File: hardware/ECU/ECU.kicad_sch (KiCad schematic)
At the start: 75 parts, among them IC1 IR4427SPBF, IC2 EL357NB_TA_-G, IC3 EL357NB_TA_-G, J1 USB_B_Micro, J2 TFP09-2-12B, J3 Connector, Q1 S8050, Q2 S8050, Q3 RJP63K2, Q4 RJP63K2, SW1 RESET, SW2 EN, U1 AMS1117-3.3, U2 AMS1117-3.3, U3 CP2102N-Axx-xQFN28, U4 ESP32-WROOM-32U

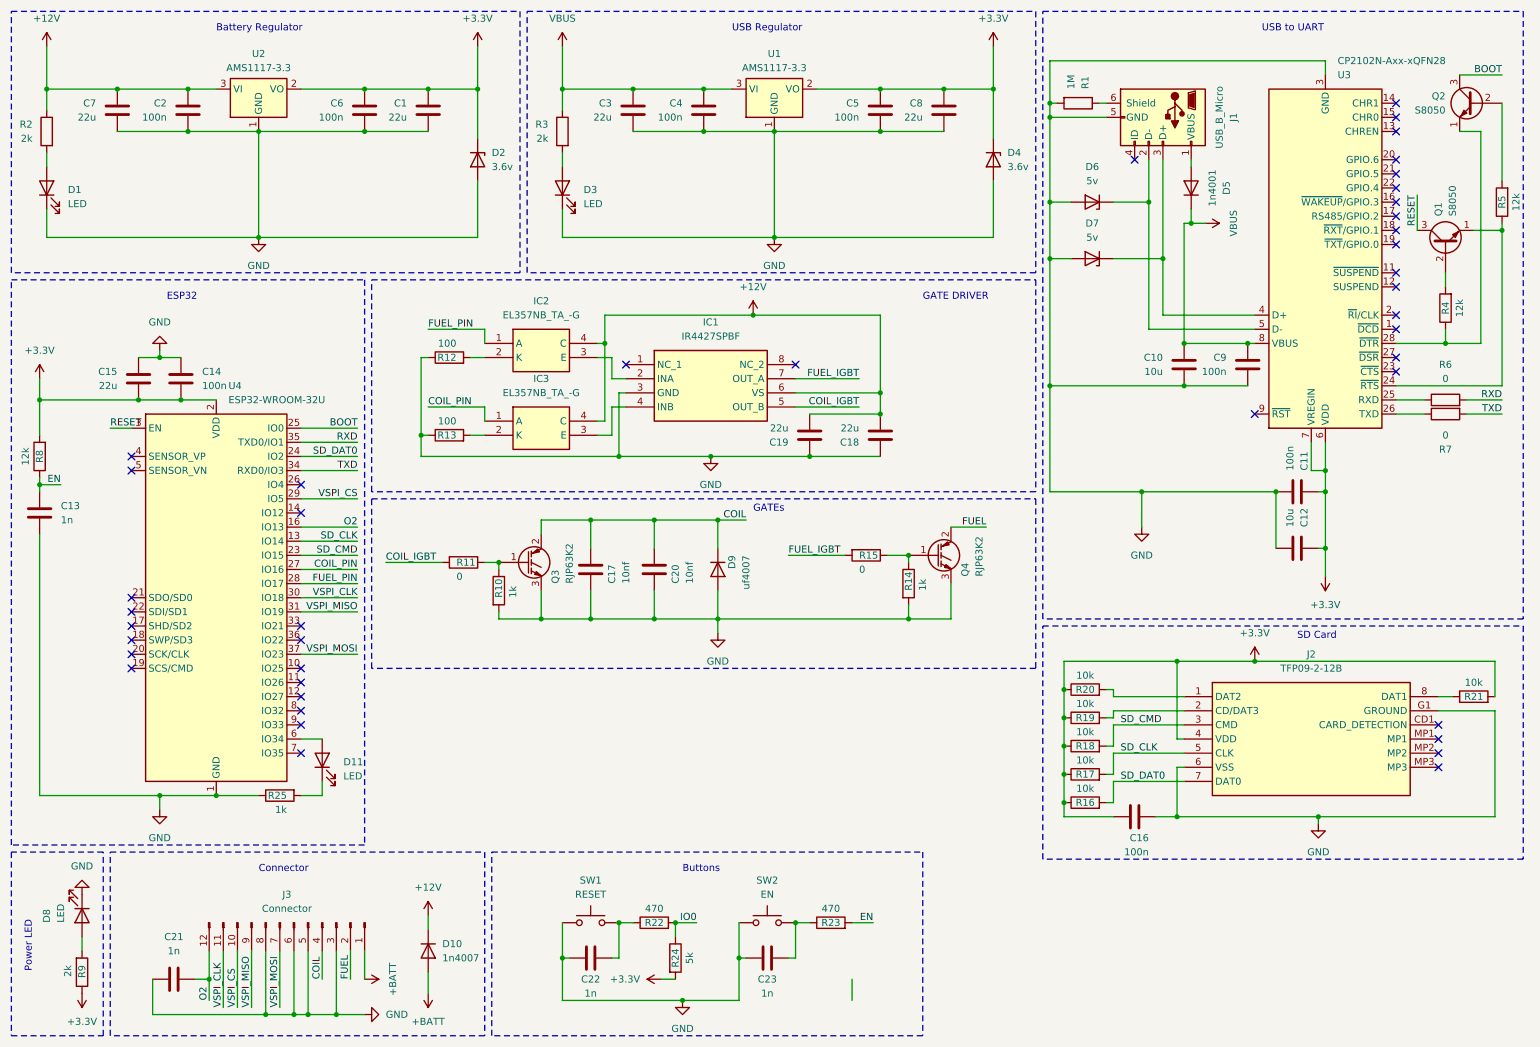
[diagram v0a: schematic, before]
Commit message: backup
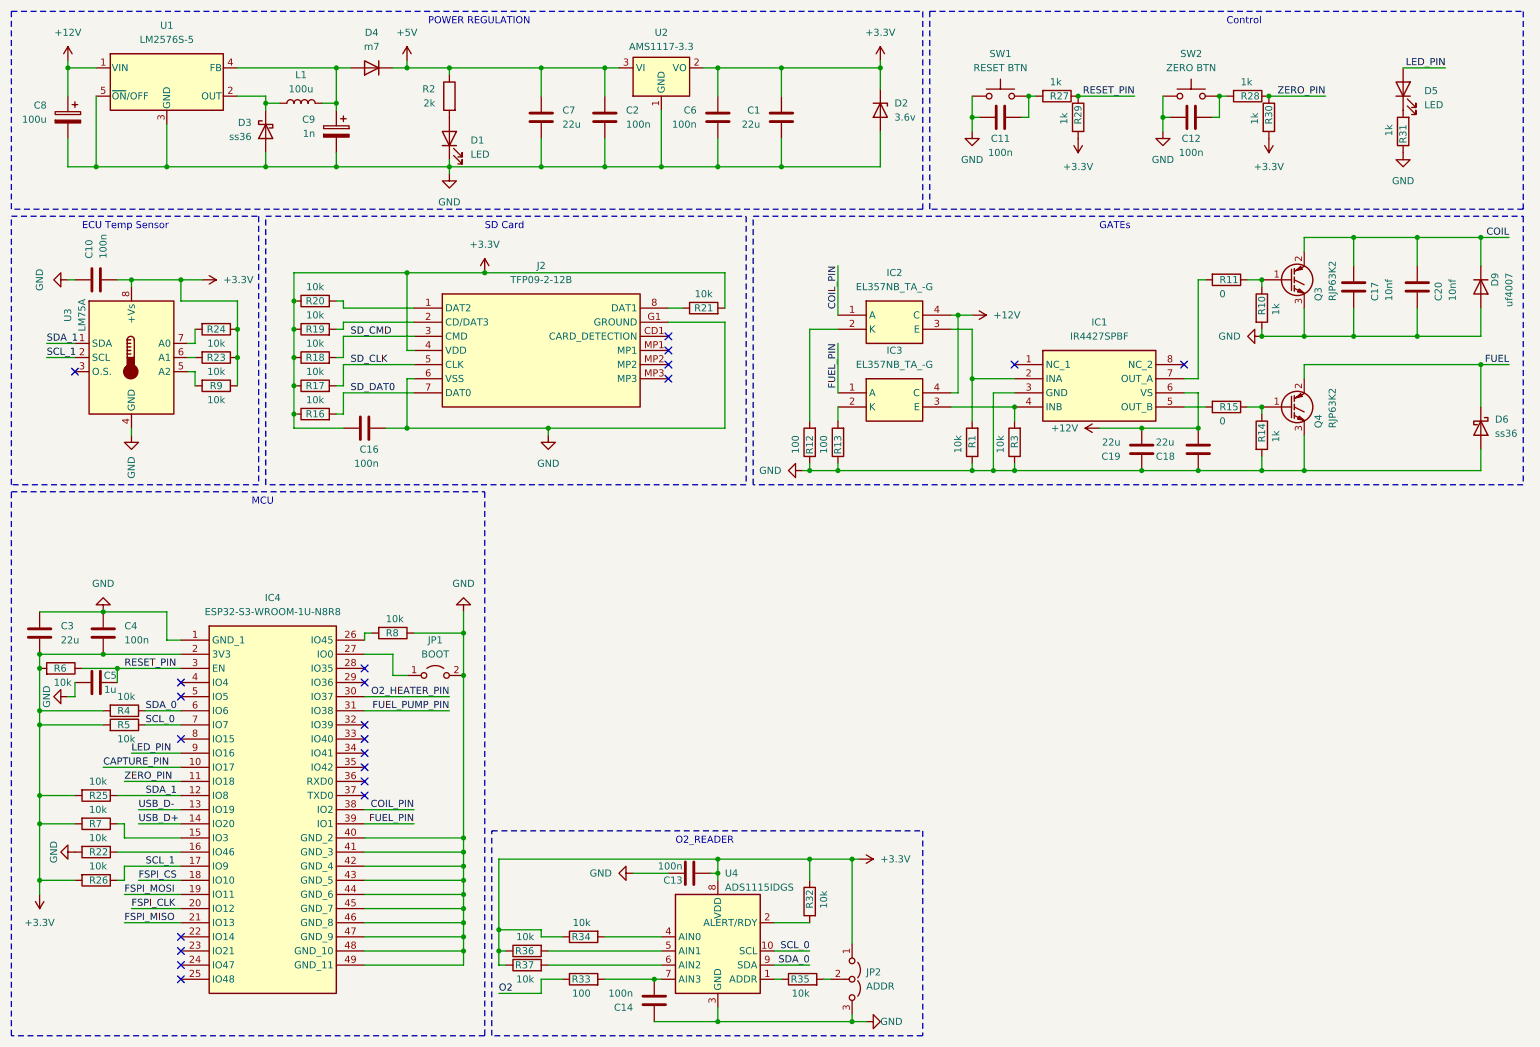
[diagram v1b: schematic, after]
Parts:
- removed C15: 22u, Capacitor_SMD:C_0603_1608Metric_Pad1.08x0.95mm_HandSolder, symbol Device:C
- removed C21, C22, C23: 1n, Capacitor_SMD:C_0603_1608Metric_Pad1.08x0.95mm_HandSolder, symbol Device:C
- removed C8: 22u, Capacitor_SMD:C_0805_2012Metric_Pad1.18x1.45mm_HandSolder, symbol Device:C
- removed C9: 100n, Capacitor_SMD:C_0603_1608Metric_Pad1.08x0.95mm_HandSolder, symbol Device:C
- removed D10: 1n4007, Diode_SMD:D_SMA, symbol Device:D
- removed D11, D3, D8: LED, LED_SMD:LED_0603_1608Metric_Pad1.05x0.95mm_HandSolder, symbol Device:LED
- removed D4: 3.6v, Diode_SMD:D_1206_3216Metric_Pad1.42x1.75mm_HandSolder, symbol Device:D_Zener
- removed D5: 1n4001, Diode_SMD:D_SMA, symbol Device:D
- removed D6, D7: 5v, Diode_SMD:D_SOD-523, symbol Device:D_Zener
- removed J1: USB_B_Micro, Connector_USB:USB_Micro-B_Molex-105017-0001, symbol Connector:USB_B_Micro
- removed J3: Connector, Connector_PinHeader_2.54mm:PinHeader_2x06_P2.54mm_Vertical, symbol Connector:Conn_01x12_Pin
- removed Q1, Q2: S8050, Package_TO_SOT_SMD:SOT-23, symbol Transistor_BJT:S8050
- removed U1: AMS1117-3.3, Package_TO_SOT_SMD:SOT-223-3_TabPin2, symbol Regulator_Linear:AMS1117-3.3
- removed U3: CP2102N-Axx-xQFN28, Package_DFN_QFN:QFN-28-1EP_5x5mm_P0.5mm_EP3.35x3.35mm, symbol Interface_USB:CP2102N-Axx-xQFN28
- removed U4: ESP32-WROOM-32U, RF_Module:ESP32-WROOM-32U, symbol RF_Module:ESP32-WROOM-32U
- added C8: 100u, Capacitor_SMD:CP_Elec_10x10, symbol Device:C_Polarized
- added C9: 1n, Capacitor_SMD:CP_Elec_10x10, symbol Device:C_Polarized
- added D3, D6: ss36, Diode_SMD:D_SMC, symbol Device:D_Schottky
- added D4: m7, Diode_SMD:D_SMA, symbol Device:D
- added D5: LED, LED_SMD:LED_0603_1608Metric_Pad1.05x0.95mm_HandSolder, symbol Device:LED
- added IC4: ESP32-S3-WROOM-1U-N8R8, ESP32S3WROOM1UN8R8, symbol My_Library:ESP32-S3-WROOM-1U-N8R8
- added JP1: BOOT, Connector_PinHeader_2.54mm:PinHeader_1x02_P2.54mm_Vertical, symbol Jumper:Jumper_2_Open
- added JP2: ADDR, Connector_PinHeader_2.54mm:PinHeader_1x03_P2.54mm_Vertical, symbol Jumper:Jumper_3_Open
- added L1: 100u, My_Lirbrary:INDPM102100X400N, symbol Device:L
- added R26, R32, R34, R35, R36, R37: 10k, Resistor_SMD:R_0603_1608Metric_Pad0.98x0.95mm_HandSolder, symbol Device:R
- added R27, R28, R29, R30, R31: 1k, Resistor_SMD:R_0603_1608Metric_Pad0.98x0.95mm_HandSolder, symbol Device:R
- added R33: 100, Resistor_SMD:R_0603_1608Metric_Pad0.98x0.95mm_HandSolder, symbol Device:R
- added U1: LM2576S-5, Package_TO_SOT_SMD:TO-263-5_TabPin3, symbol Regulator_Switching:LM2576S-5
- added U3: LM75A, symbol Sensor_Temperature:LM75B
- added U4: ADS1115IDGS, Package_SO:TSSOP-10_3x3mm_P0.5mm, symbol Analog_ADC:ADS1115IDGS
- C10: value 10u -> 100n; footprint Capacitor_SMD:C_0603_1608Metric_Pad1.08x0.95mm_HandSolder -> Capacitor_SMD:C_0805_2012Metric_Pad1.18x1.45mm_HandSolder
- C11, C14: footprint Capacitor_SMD:C_0603_1608Metric_Pad1.08x0.95mm_HandSolder -> Capacitor_SMD:C_0603_1608Metric
- C12: value 10u -> 100n; footprint Capacitor_SMD:C_0603_1608Metric_Pad1.08x0.95mm_HandSolder -> Capacitor_SMD:C_0603_1608Metric
- C13: value 1n -> 100n; footprint Capacitor_SMD:C_0603_1608Metric_Pad1.08x0.95mm_HandSolder -> Capacitor_SMD:C_0603_1608Metric
- C3, C4: footprint Capacitor_SMD:C_0805_2012Metric_Pad1.18x1.45mm_HandSolder -> Capacitor_SMD:C_0603_1608Metric
- C5: value 100n -> 1u; footprint Capacitor_SMD:C_0805_2012Metric_Pad1.18x1.45mm_HandSolder -> Capacitor_SMD:C_0603_1608Metric
- R1: value 1M -> 10k
- R22, R23: value 470 -> 10k
- R24: value 5k -> 10k
- R25: value 1k -> 10k
- R3, R9: value 2k -> 10k
- R4, R5, R8: value 12k -> 10k
- R6, R7: value 0 -> 10k
- SW1: value RESET -> RESET BTN; footprint Button_Switch_SMD:SW_Push_1P1T_NO_CK_KMR2 -> Button_Switch_SMD:SW_SPST_PTS810
- SW2: value EN -> ZERO BTN; footprint Button_Switch_SMD:SW_Push_1P1T_NO_CK_KMR2 -> Button_Switch_SMD:SW_SPST_PTS810
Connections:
- net RXD is gone; now on net +3.3V: R6.2
- net TXD is gone; now on net +3.3V: R7.2
- net VBUS is gone; now on net GND: C10.1, C3.1, C4.1, R3.1
- net +12V: now also C8.1, U1.1 (VIN); no longer C2.1, C7.1, R2.1, U2.3 (VI)
- net +3.3V: now also C10.2, C13.2, C3.2, C4.2, R23.1, R24.1, R25.2, R4.2, R5.2, IC4.2 (3V3), JP2.1 (A), R26.2, R29.2, R30.2, R32.1, R34.1, R36.1, R37.1, U3.8 (+Vs), U4.8 (VDD); no longer C11.1, C12.1, C14.2, C5.1, R24.2, R8.2
- net COIL_PIN: now also IC2.1 (A), IC4.38 (IO2); no longer IC3.1 (A)
- net FUEL: now also D6.1 (K)
- net FUEL_PIN: now also IC3.1 (A), IC4.39 (IO1); no longer IC2.1 (A)
- net GND: now also C11.1, C12.1, C13.1, C5.1, R1.1, R22.2, R8.1, C8.2, C9.2, D3.2 (A), D6.2 (A), IC4.1 (GND_1), IC4.40 (GND_2), IC4.41 (GND_3), IC4.42 (GND_4), IC4.43 (GND_5), IC4.44 (GND_6), IC4.45 (GND_7), IC4.46 (GND_8), IC4.47 (GND_9), IC4.48 (GND_10), IC4.49 (GND_11), JP1.2 (B), JP2.3 (B), R31.1, U1.3 (GND), U1.5 (~{ON}/OFF), U3.4 (GND), U4.3 (GND); no longer C10.2, C11.2, C12.2, C13.2, C3.2, C4.2, C5.2, R1.2, R25.1
- net O2: now also R33.1
- net at R3.2: now also IC1.4 (INB), IC3.3 (E)
- net at R22.1: now also IC4.16 (IO46); no longer SW1.2
- net at R7.1: now also IC4.15 (IO3)
- net SCL_0: now reaches R5.1
- net SCL_0: now also IC4.7 (IO7), U4.10 (SCL)
- net at R9.2: now also U3.5 (A2)
- net at SW2.2: now also C12.2, R28.2; no longer R23.1
- net at IC1.2 (INA), IC2.3 (E): now also R1.2
- net RESET_PIN: now reaches R6.1
- net RESET_PIN: now also C5.2, IC4.3 (EN), R27.1, R29.1
- net SDA_0: now reaches R4.1
- net SDA_0: now also IC4.6 (IO6), U4.9 (SDA)
- net COIL_IGBT: no longer names the net of IC1.5 (OUT_B)
- net COIL_IGBT: now also R15.2; no longer R11.2
- removed net EN: C13.1, R23.2, R8.1
- net FUEL_IGBT: no longer names the net of IC1.7 (OUT_A)
- net FUEL_IGBT: now also R11.2; no longer R15.2
- removed net IO0: R22.2, R24.1
- new net: D3.1 (K), L1.1, U1.2 (OUT)
- new net: C9.1, D4.2 (A), L1.2, U1.4 (FB)
- new net: IC4.26 (IO45), R8.2
- new net: IC4.27 (IO0), JP1.1 (A)
- new net: R35.1, U4.1 (ADDR)
- new net: JP2.2 (C), R35.2
- new net: R37.2, U4.6 (AIN2)
- new net: C11.2, R27.2, SW1.2
- new net: R23.2, U3.6 (A1)
- new net: D5.1 (K), R31.2
- new net: R24.2, U3.7 (A0)
- new net: R36.2, U4.5 (AIN1)
- new net: C14.2, R33.2, U4.7 (AIN3)
- new net: R34.2, U4.4 (AIN0)
- new net: R32.2, U4.2 (ALERT/RDY)
- new net +5V: C2.1, C7.1, D4.1 (K), R2.1, U2.3 (VI)
- new net CAPTURE_PIN: IC4.10 (IO17)
- new net FSPI_CLK: IC4.20 (IO12)
- new net FSPI_CS: IC4.18 (IO10)
- new net FSPI_MISO: IC4.21 (IO13)
- new net FSPI_MOSI: IC4.19 (IO11)
- new net FUEL_PUMP_PIN: IC4.31 (IO38)
- new net LED_PIN: D5.2 (A), IC4.9 (IO16)
- new net O2_HEATER_PIN: IC4.30 (IO37)
- new net SCL_1: IC4.17 (IO9), R26.1, U3.2 (SCL)
- new net SDA_1: IC4.12 (IO8), R25.1, U3.1 (SDA)
- new net USB_D+: IC4.14 (IO20)
- new net USB_D-: IC4.13 (IO19)
- new net ZERO_PIN: IC4.11 (IO18), R28.1, R30.1
- no-connect marks 42 -> 22
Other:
- note added: "Control"
- note added: "ECU Temp Sensor"
- note added: "MCU"
- note added: "O2_READER"
- note added: "POWER REGULATION"
- note removed: "Battery Regulator"
- note removed: "Buttons"
- note removed: "Connector"
- note removed: "ESP32"
- note removed: "GATE DRIVER"
- note removed: "Power LED"
- note removed: "USB Regulator"
- note removed: "USB to UART"
- moved on the sheet: C1, C16, C17, C18, C19, C2, C20, C6, C7, D1, D2, D9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

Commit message: ECU hardware v0.2 candidate
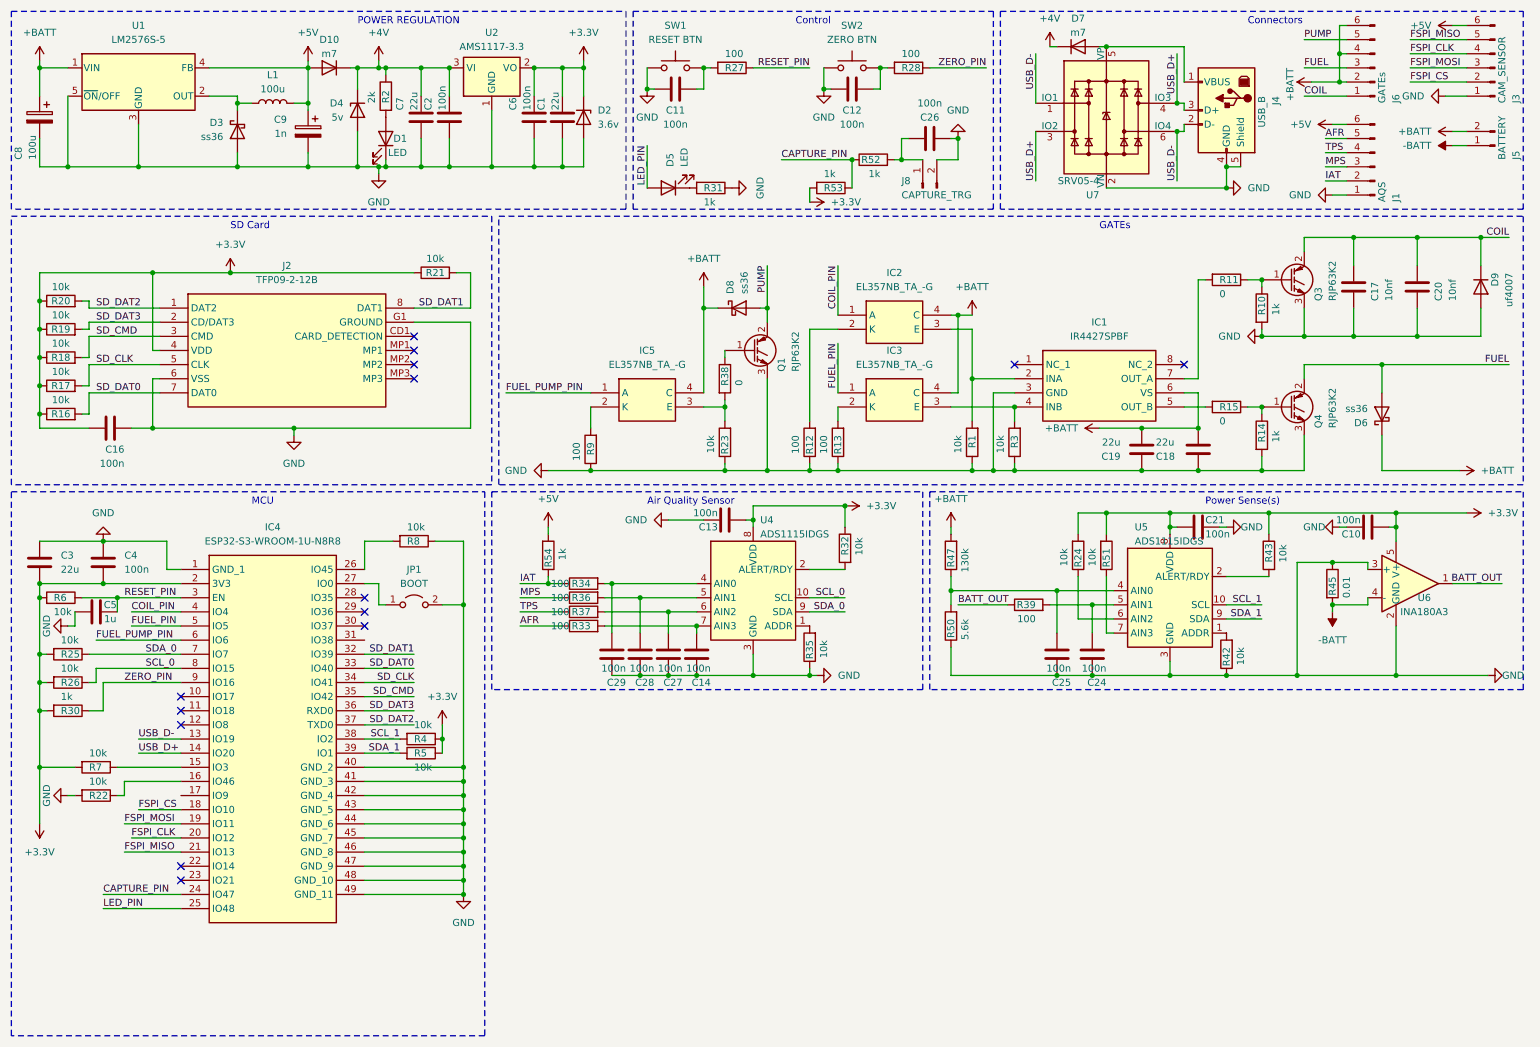
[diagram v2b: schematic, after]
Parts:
- removed D4: m7, Diode_SMD:D_SMA, symbol Device:D
- removed JP2: ADDR, Connector_PinHeader_2.54mm:PinHeader_1x03_P2.54mm_Vertical, symbol Jumper:Jumper_3_Open
- removed R29: 1k, Resistor_SMD:R_0603_1608Metric_Pad0.98x0.95mm_HandSolder, symbol Device:R
- removed U3: LM75A, symbol Sensor_Temperature:LM75B
- added C21, C24, C25, C26, C27, C28, C29: 100n, Capacitor_SMD:C_0603_1608Metric, symbol Device:C
- added D10, D7: m7, Diode_SMD:D_SMA, symbol Device:D
- added D4: 5v, Diode_SMD:D_1206_3216Metric_Pad1.42x1.75mm_HandSolder, symbol Device:D_Zener
- added D8: ss36, Diode_SMD:D_SMC, symbol Device:D_Schottky
- added IC5: EL357NB_TA_-G, MyLibrary:EL357NG, symbol My_Library:EL357NB_TA_-G
- added J1: AQS, Connector_JST:JST_XH_B6B-XH-A_1x06_P2.50mm_Vertical, symbol Connector:Conn_01x06_Pin
- added J3: CAM_SENSOR, Connector_JST:JST_XH_B6B-XH-A_1x06_P2.50mm_Vertical, symbol Connector:Conn_01x06_Pin
- added J4: USB_B, Connector_USB:USB_B_TE_5787834_Vertical, symbol Connector:USB_B
- added J5: BATTERY, Connector_Molex:Molex_KK-396_5273-02A_1x02_P3.96mm_Vertical, symbol Connector:Conn_01x02_Pin
- added J6: GATEs, Connector_Molex:Molex_KK-396_5273-06A_1x06_P3.96mm_Vertical, symbol Connector:Conn_01x06_Pin
- added J8: CAPTURE_TRG, Connector_JST:JST_XH_B2B-XH-A_1x02_P2.50mm_Vertical, symbol Connector:Conn_01x02_Pin
- added Q1: RJP63K2, Package_TO_SOT_SMD:TO-263-2, symbol Device:Q_NIGBT_GCE
- added R38: 0, Resistor_SMD:R_0603_1608Metric_Pad0.98x0.95mm_HandSolder, symbol Device:R
- added R39: 100, Resistor_SMD:R_0603_1608Metric_Pad0.98x0.95mm_HandSolder, symbol Device:R
- added R42, R43, R51: 10k, Resistor_SMD:R_0603_1608Metric_Pad0.98x0.95mm_HandSolder, symbol Device:R
- added R45: 0.01, MyLibrary:RESC10052X106N, symbol Device:R
- added R47: 130k, Resistor_SMD:R_0603_1608Metric_Pad0.98x0.95mm_HandSolder, symbol Device:R
- added R50: 5.6k, Resistor_SMD:R_0603_1608Metric_Pad0.98x0.95mm_HandSolder, symbol Device:R
- added R52, R53, R54: 1k, Resistor_SMD:R_0603_1608Metric_Pad0.98x0.95mm_HandSolder, symbol Device:R
- added U5: ADS1115IDGS, Package_SO:TSSOP-10_3x3mm_P0.5mm, symbol Analog_ADC:ADS1115IDGS
- added U6: INA180A3, Package_TO_SOT_SMD:SOT-23-5, symbol Amplifier_Current:INA180A3
- added U7: SRV05-4, Package_TO_SOT_SMD:SOT-23-6, symbol Power_Protection:SRV05-4
- C10: footprint Capacitor_SMD:C_0805_2012Metric_Pad1.18x1.45mm_HandSolder -> Capacitor_SMD:C_0603_1608Metric
- IC1: footprint My_Lirbrary:SOIC127P600X175-8N -> MyLibrary:SOIC127P600X175-8N
- IC2, IC3: footprint SOP254P700X200-4N -> MyLibrary:EL357NG
- IC4: footprint ESP32S3WROOM1UN8R8 -> MyLibrary:ESP32S3WROOM1UN4
- J2: footprint TFP09212B -> MyLibrary:TFP09212B
- L1: footprint My_Lirbrary:INDPM102100X400N -> MyLibrary:INDPM102100X400N
- R16, R17, R18, R19, R20, R21: footprint Resistor_SMD:R_0603_1608Metric_Pad0.98x0.95mm_HandSolder -> Resistor_SMD:R_0603_1608Metric
- R27, R28: value 1k -> 100
- R34, R36, R37, R9: value 10k -> 100
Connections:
- net +3.3V: now also R21.1, R24.2, R4.1, R5.1, C21.2, R43.1, R51.2, R53.2, U5.8 (VDD), U6.5 (V+); no longer R21.2, R23.1, R24.1, R34.1, R36.1, R37.1, R4.2, R5.2, R9.1
- net +5V: now also C9.1, L1.2, U1.4 (FB), D10.2 (A), J1.6 (Pin_6), J3.6 (Pin_6), R54.2; no longer C2.1, C7.1, R2.1, U2.3 (VI)
- net CAPTURE_PIN: now also IC4.24 (IO47), R52.1, R53.1; no longer IC4.10 (IO17)
- net COIL: now also J6.1 (Pin_1)
- net COIL_PIN: now also IC4.4 (IO4); no longer IC4.38 (IO2)
- net FSPI_CLK: now also J3.4 (Pin_4)
- net FSPI_CS: now also J3.2 (Pin_2)
- net FSPI_MISO: now also J3.5 (Pin_5)
- net FSPI_MOSI: now also J3.3 (Pin_3)
- net FUEL: now also D6.2 (A), J6.3 (Pin_3); no longer D6.1 (K)
- net FUEL_PIN: now also IC4.5 (IO5); no longer IC4.39 (IO1)
- net FUEL_PUMP_PIN: now also IC4.6 (IO6), IC5.1 (A); no longer IC4.31 (IO38)
- net GND: now also R23.1, R35.1, R9.1, C21.1, C24.1, C25.1, C26.1, C27.1, C28.1, C29.1, D4.2 (A), J1.1 (Pin_1), J3.1 (Pin_1), J4.4 (GND), J4.5 (Shield), J8.2 (Pin_2), Q1.3 (E), R42.1, R45.1, R50.1, U5.3 (GND), U6.2 (GND), U6.3 (+), U7.2 (VN); no longer D6.2 (A)
- net LED_PIN: now also IC4.25 (IO48); no longer IC4.9 (IO16)
- net SCL_0: now also IC4.8 (IO15), R26.1; no longer IC4.7 (IO7), R5.1
- net SCL_1: now also IC4.38 (IO2), R4.2, U5.10 (SCL); no longer IC4.17 (IO9), R26.1
- net SDA_0: now also IC4.7 (IO7), R25.1; no longer IC4.6 (IO6), R4.1
- net SDA_1: now also IC4.39 (IO1), R5.2, U5.9 (SDA); no longer IC4.12 (IO8), R25.1
- net SD_CLK: now also IC4.34 (IO41)
- net SD_CMD: now also IC4.35 (IO42)
- net SD_DAT0: now also IC4.33 (IO40)
- net USB_D+: now also J4.3 (D+), U7.3 (IO2), U7.4 (IO3)
- net USB_D-: now also J4.2 (D-), U7.1 (IO1), U7.6 (IO4)
- net ZERO_PIN: now also IC4.9 (IO16); no longer IC4.11 (IO18)
- net at R9.2: now also IC5.2 (K)
- net SD_DAT1: now reaches IC4.32 (IO39)
- net SD_DAT1: now also J2.8 (DAT1), R21.2
- net SD_DAT3: now reaches IC4.36 (RXD0)
- net SD_DAT3: now also J2.2 (CD/DAT3), R19.2
- net SD_DAT2: now reaches IC4.37 (TXD0)
- net SD_DAT2: now also J2.1 (DAT2), R20.2
- net at U4.1 (ADDR): now also R35.2; no longer R35.1
- net at R37.2, U4.6 (AIN2): now also C27.2
- net at R23.2: now also IC5.3 (E), R38.2
- net at R36.2, U4.5 (AIN1): now also C28.2
- net at R34.2, U4.4 (AIN0): now also C29.2
- net +12V renamed +BATT
- net +BATT: now also D6.1 (K), D8.1 (K), IC5.4 (C), J5.2 (Pin_2), J6.2 (Pin_2), J6.4 (Pin_4), J6.6 (Pin_6), R47.2
- net O2 renamed AFR
- net AFR: now also J1.5 (Pin_5)
- net O2_HEATER_PIN: no longer names the net of IC4.30 (IO37)
- new net: C25.2, R47.1, R50.2, U5.4 (AIN0)
- new net: C24.2, R39.2, U5.5 (AIN1)
- new net: D7.2 (A), J4.1 (VBUS), U7.5 (VP)
- new net: R24.1, U5.6 (AIN2)
- new net: R43.2, U5.2 (ALERT/RDY)
- new net: C26.2, J8.1 (Pin_1), R52.2
- new net: Q1.1 (G), R38.1
- new net: R42.2, U5.1 (ADDR)
- new net: R51.1, U5.7 (AIN3)
- new net +4V: C2.1, C7.1, D10.1 (K), D4.1 (K), D7.1 (K), R2.1, U2.3 (VI)
- new net -BATT: J5.1 (Pin_1), R45.2, U6.4 (-)
- new net BATT_OUT: R39.1, U6.1
- new net IAT: J1.2 (Pin_2), R34.1, R54.1
- new net MPS: J1.3 (Pin_3), R36.1
- new net PUMP: D8.2 (A), J6.5 (Pin_5), Q1.2 (C)
- new net TPS: J1.4 (Pin_4), R37.1
- no-connect marks 22 -> 14
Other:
- note added: "Air Quality Sensor"
- note added: "Connectors"
- note added: "Power Sense(s)"
- note removed: "ECU Temp Sensor"
- note removed: "O2_READER"
- moved on the sheet: C1, C11, C12, C13, C14, C16, C2, C3, C4, C5, C6, C7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
